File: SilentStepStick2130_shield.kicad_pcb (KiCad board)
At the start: 4 copper layers, 68.6 x 53.3 mm, 11 parts, among them J1 Conn_01x04_Socket, J2 Conn_01x04_Socket, J3 Conn_01x02_Pin, J4 Conn_01x02_Pin, J5 Conn_01x03, J6 Conn_01x02_Pin, U1 TMC2130_SILENTSTEPSTICK, U2 TMC2130_SILENTSTEPSTICK

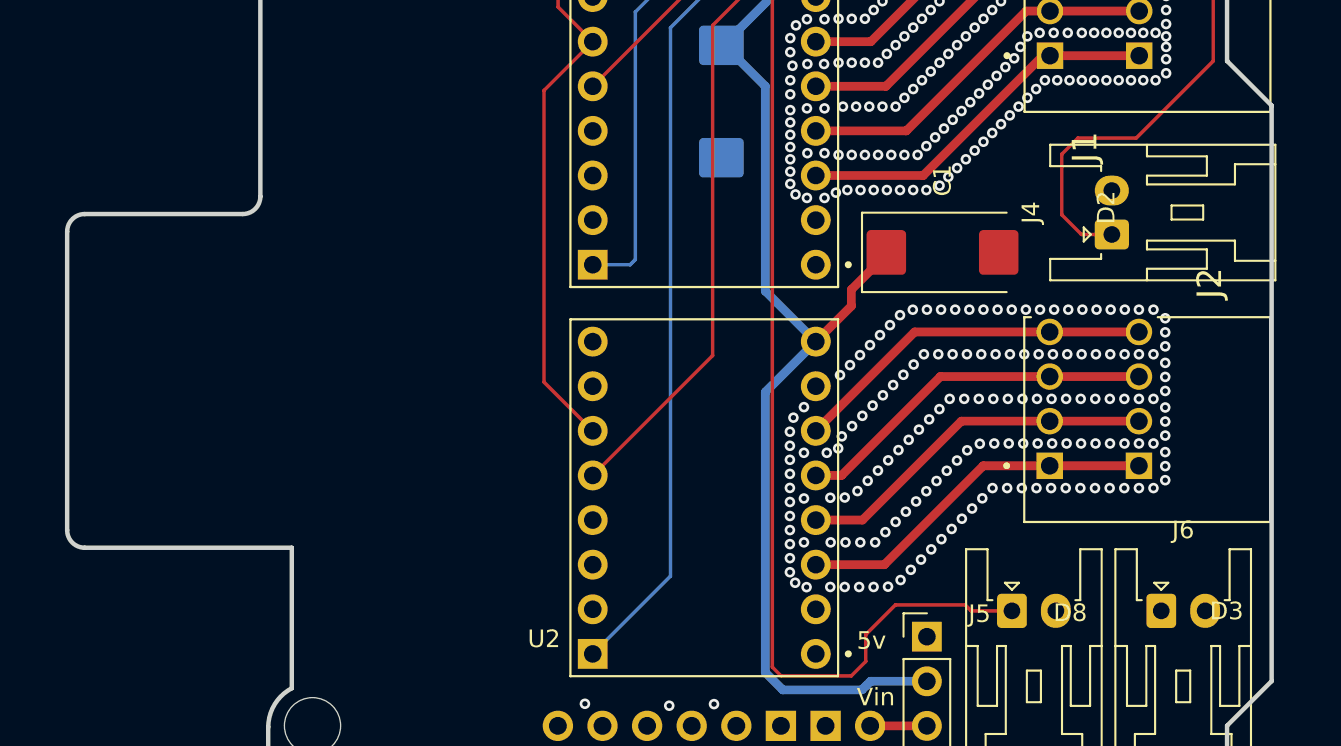
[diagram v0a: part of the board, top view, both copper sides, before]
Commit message: v4
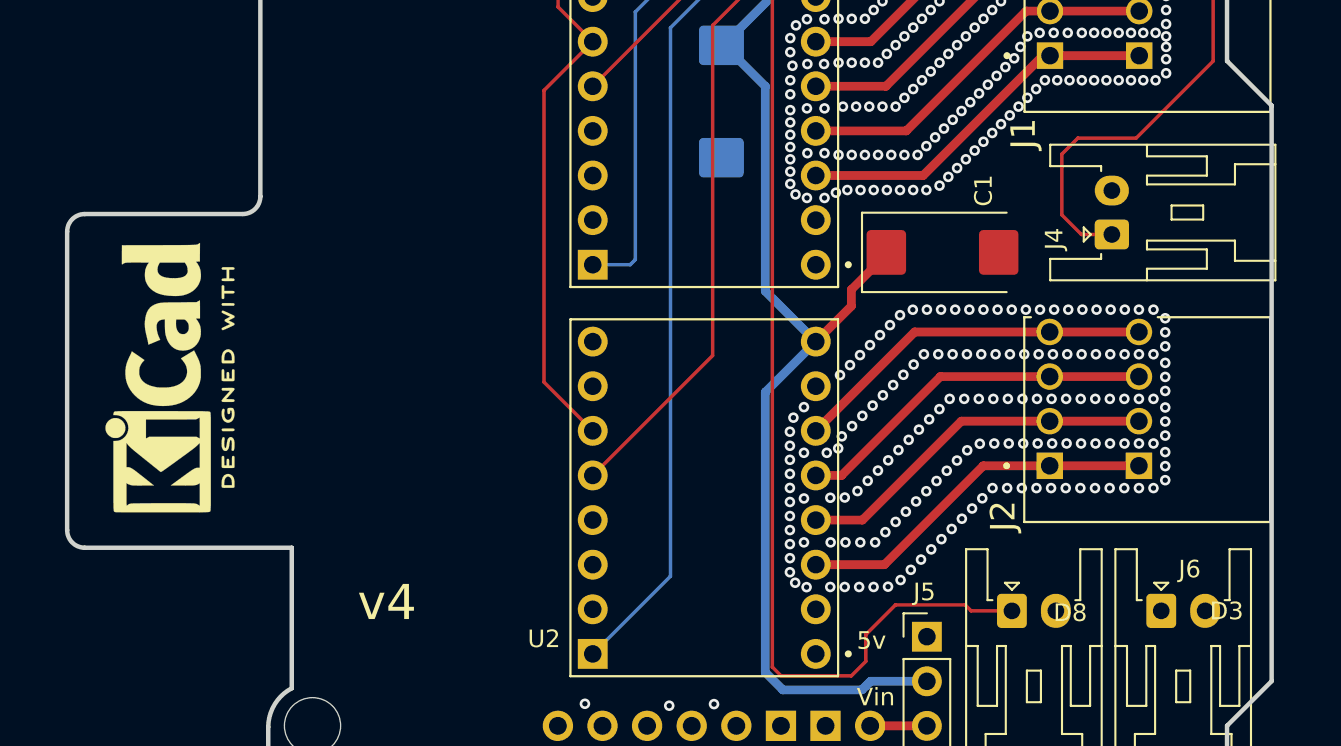
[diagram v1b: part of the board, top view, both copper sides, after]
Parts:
- added REF**: KiCad-Logo2_6mm_SilkScreen, Symbol:KiCad-Logo2_6mm_SilkScreen, F.Cu at (112.4, 79.9)
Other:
- board text added: "v4"
- board text removed: "D2"
